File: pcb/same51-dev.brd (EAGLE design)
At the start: 83.5 x 68.2 mm, 61 parts, among them J1 4, J10 8, J11 2, J2 USB-C, J3 6, J4 8, J5 8, J6 3, J7 8, J8 8, J9 5, SW2 MSK-13C01, U1 ATSAMD51J, U2 W25Q40BVSS, U3 MCP1631TDFN8, U4 MCP2562-MF, X1 32.768kHz

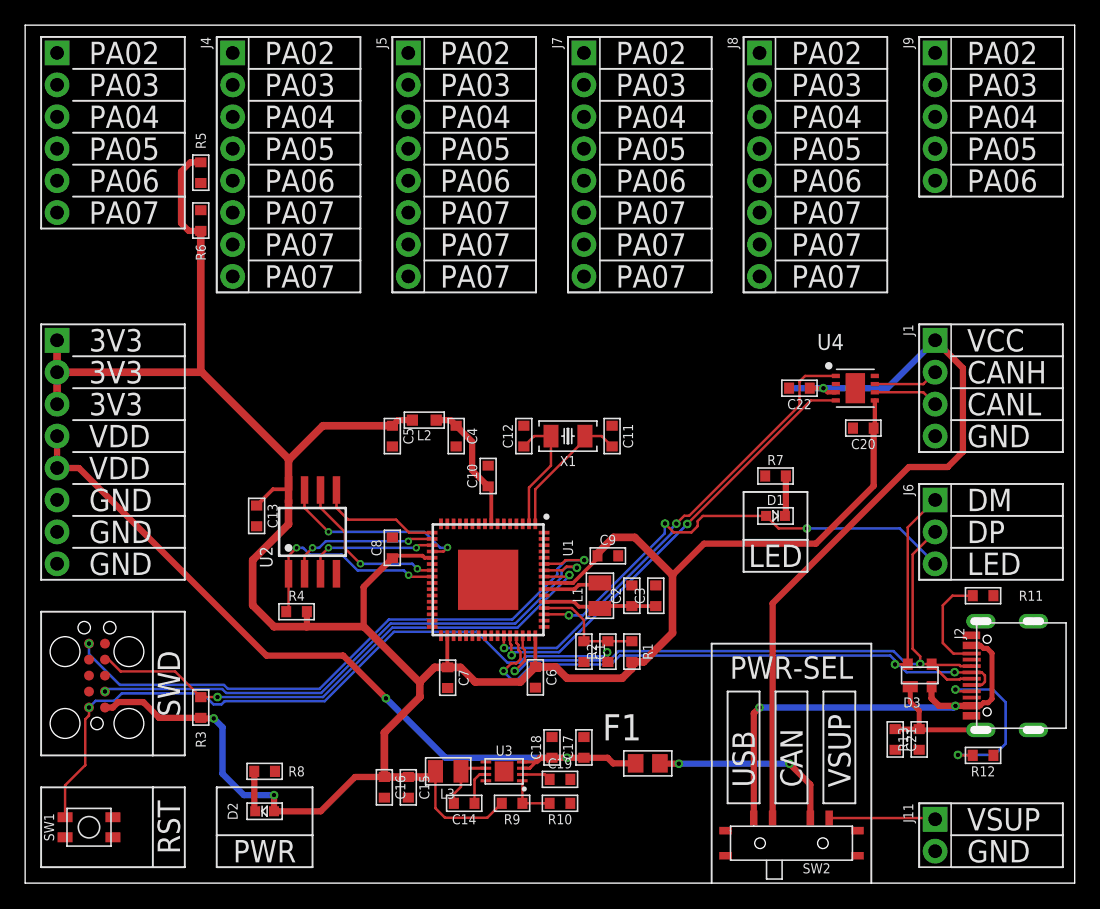
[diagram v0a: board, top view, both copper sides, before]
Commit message: finished signal routing
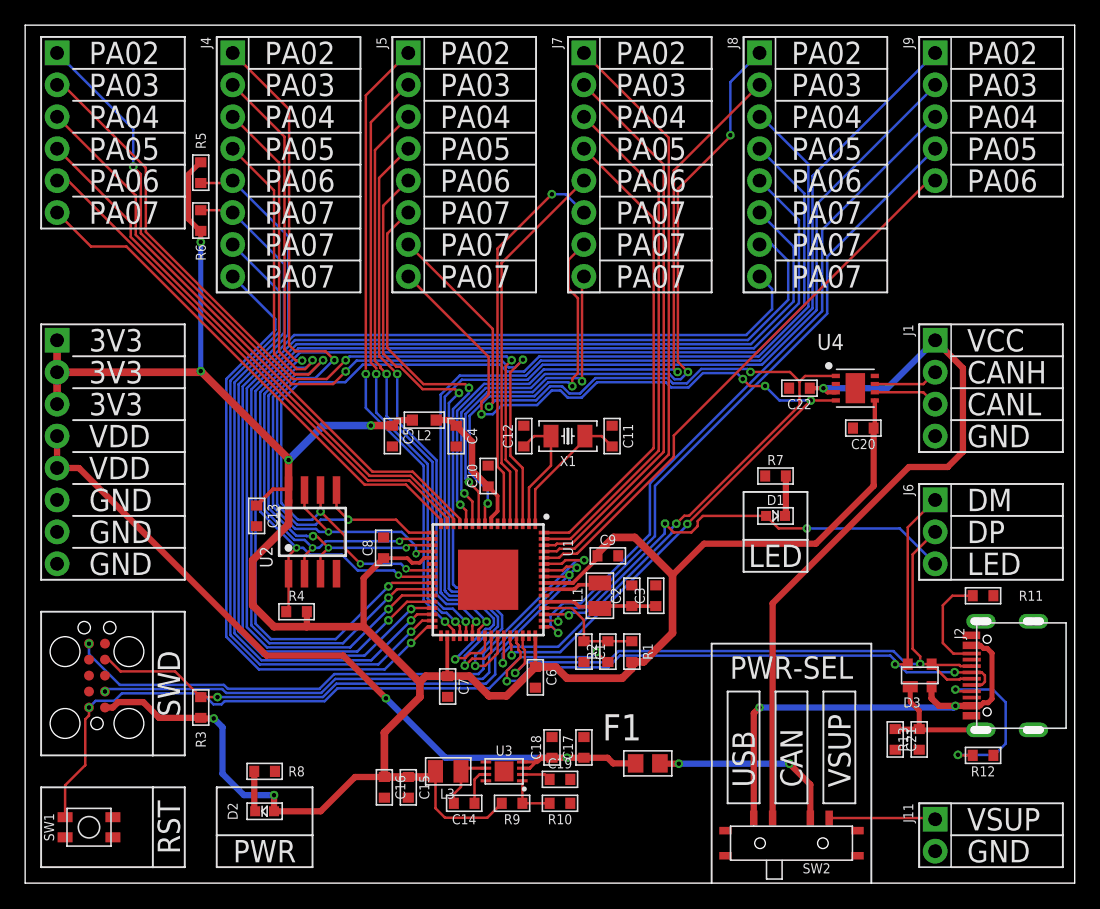
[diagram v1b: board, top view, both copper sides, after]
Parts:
- moved C7 0.70 mm to (33.6, 15.6)
- moved C8 0.70 mm to (28.5, 26.7)
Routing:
- net PB12: track 0.00 -> 92.1 mm, vias 0 -> 1
- net PB13: track 0.00 -> 89.7 mm, vias 0 -> 1
- net PB14: track 0.00 -> 88.0 mm, vias 0 -> 1
- net PB15: track 0.00 -> 84.5 mm, vias 0 -> 1
- net PB17: track 0.00 -> 83.0 mm, vias 0 -> 1
- net PB16: track 0.00 -> 78.5 mm, vias 0 -> 1
- net QSPI_SCK: track 13.1 -> 87.5 mm, vias 2 -> 3
- net QSPI_CS: track 17.2 -> 90.8 mm
- net PA02: track 0.00 -> 67.6 mm, vias 0 -> 3
- net PA03: track 0.00 -> 63.3 mm, vias 0 -> 2
- net SDA: track 0.00 -> 59.7 mm, vias 0 -> 1
- net SCL: track 0.00 -> 57.5 mm, vias 0 -> 1
- net PB08: track 0.00 -> 57.3 mm, vias 0 -> 3
- net PB22: track 0.00 -> 56.1 mm, vias 0 -> 1
- net PB09: track 0.00 -> 54.1 mm, vias 0 -> 2
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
